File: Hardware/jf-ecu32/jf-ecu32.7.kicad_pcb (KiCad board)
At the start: 2 copper layers, 71.3 x 48 mm, 88 parts, among them J1 GAZ, J10 k, J11 RPM, J12 S.PORT, J13 PPM/PWM, J14 PUMP1, J15 PUMP1, J16 PPM/PWM, J17 PUMP2, J18 PUMP2, J19 EN, J2 AUX, J21 Conn_01x07, J3 PPM/PWM, J4 STARTER, J5 GLOW, J6 VANNE KEROSTART, J7 VANNE KERO, J8 BATTERY 2S/3S, J9 STARTER, Q1 AO3400A, Q2 QM6006D, Q3 AO3400A, Q4 QM6006D, Q5 QM6006D, Q6 QM6006D, Q7 AO3400A, Q8 AO3400A, U1 ESP32-WROOM-32D, U2 4050, U3 MAX31855KASA, U4 AMS1117-3.3, U5 4050, U6 AMS1117-5.0, U7 OPA340NA, U8 LM4040DBZ-2.5, U9 INA219AxDCN

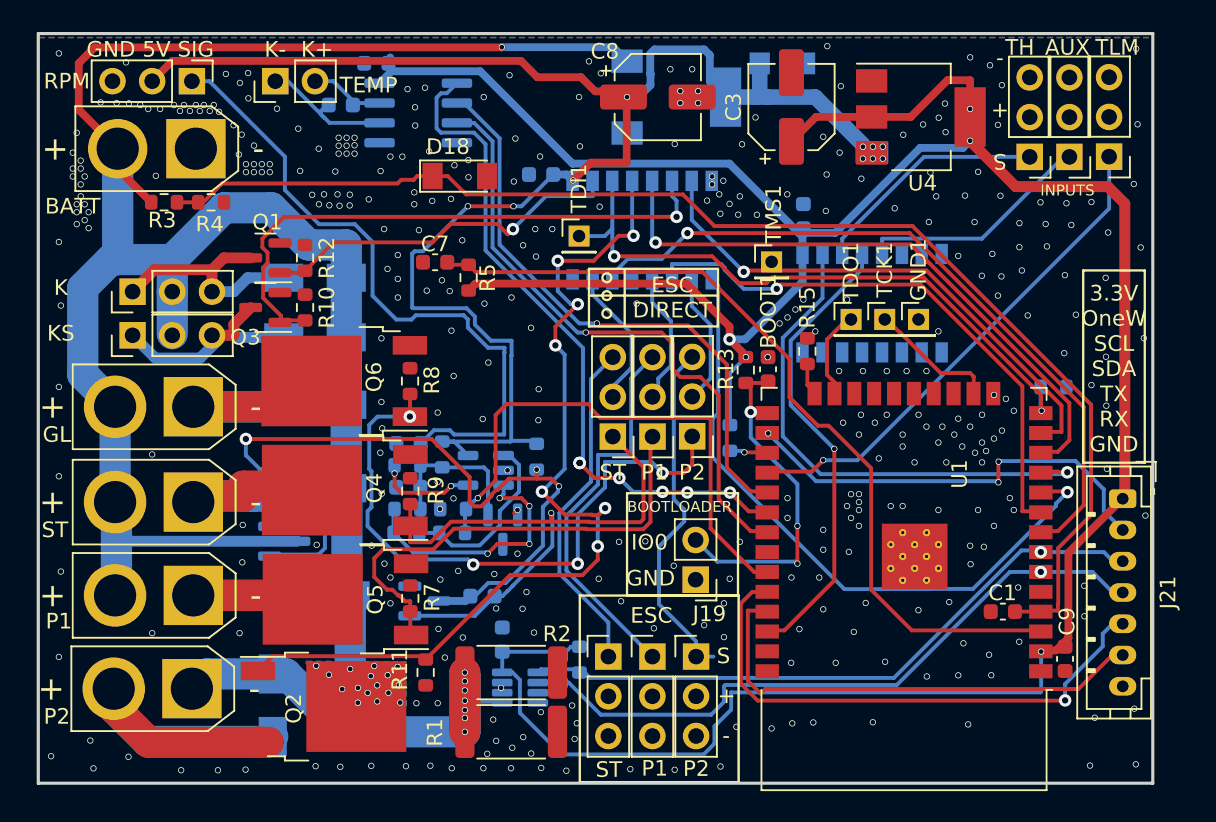
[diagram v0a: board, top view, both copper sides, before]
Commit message: PCB + SRC
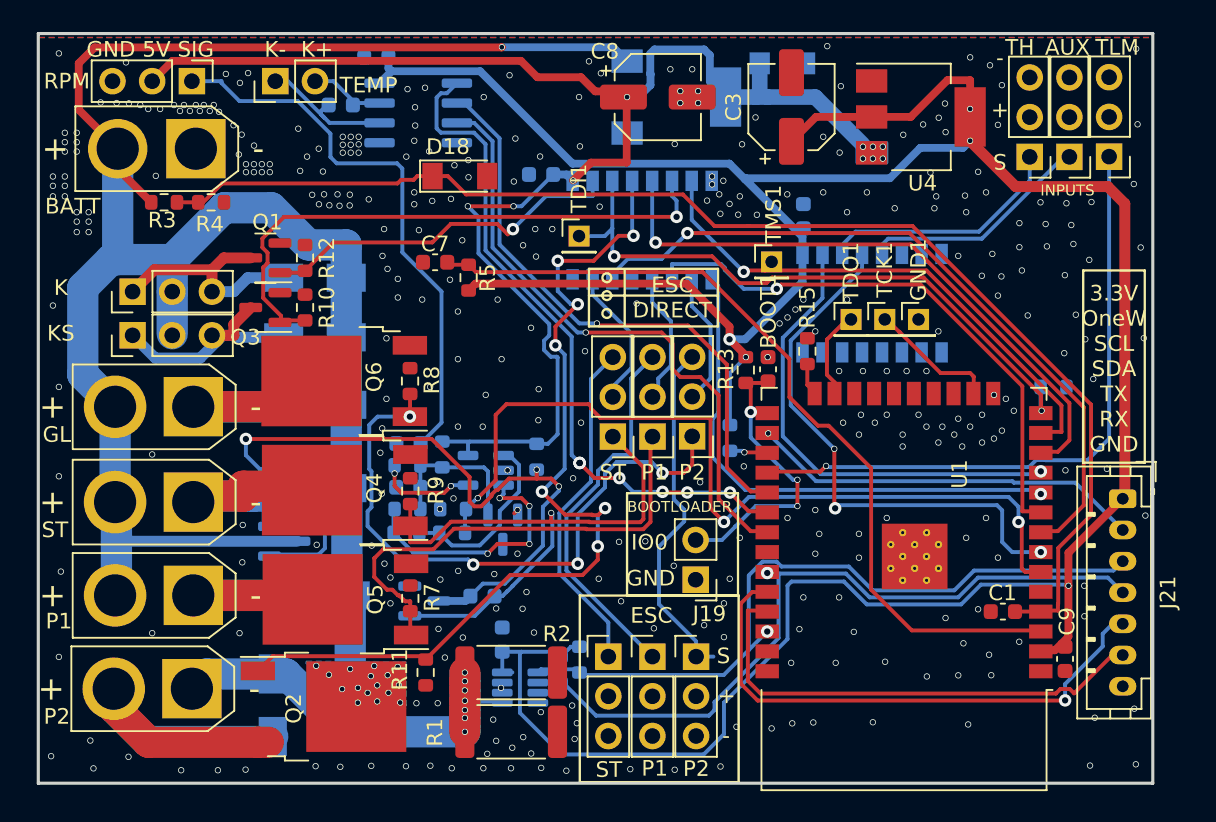
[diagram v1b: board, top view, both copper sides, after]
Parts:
- moved C11 0.38 mm to (34.4, 151.6)
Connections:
- net Net-(J13-Pin_3) renamed P1_OUTPUT
- net Net-(J16-Pin_3) renamed P2_OUTPUT
- net Net-(J3-Pin_3) renamed ST_OUTPUT
- U1 pad 33: RPM-2 -> ESP_SDA
- U1 pad 36: AUX -> ESP_SCL
- U1 pad 6: ESP_SDA -> RPM-2
- U1 pad 7: ESP_SCL -> AUX
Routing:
- net RPM-2: track 34.7 -> 54.9 mm, vias 1 -> 3
- net TX2: track 32.1 -> 40.8 mm
- net PPM_PWM_PUMP2_3.3: track 42.3 -> 33.8 mm
- net 3.3V: track 193.9 -> 202.2 mm
- net RPM: track 42.2 -> 35.9 mm
- net ESP_SCL: track 40.7 -> 46.7 mm
- net AUX: track 29.5 -> 35.0 mm, vias 1 -> 3
- net ESP_SDA: track 42.5 -> 47.1 mm
- net +5V: track 98.5 -> 94.1 mm
- net PPM_GAZ: track 33.7 -> 30.3 mm
- net IO0: track 22.5 -> 19.2 mm
- net OneWire: track 28.0 -> 25.2 mm, vias 3 -> 1
- net PPM_GAZ_5V: track 15.1 -> 15.8 mm
- net P1_OUTPUT: track 25.0 -> 24.4 mm
- net GND: vias 372 -> 355
